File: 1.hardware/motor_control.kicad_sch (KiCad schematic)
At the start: 33 parts, among them IC1 UCC27712QDRQ1, IC4 SN74HC266D, J10 MOTOR_1_UVW, J11 MOTOR_1_HALL_SENSOR, Q10 STL130N6F7, Q2 STL130N6F7, Q3 STL130N6F7, Q4 STL130N6F7, Q8 STL130N6F7, Q9 STL130N6F7, U13 IR2101, U14 IR2101, U7 LM2904D, U8 LM2904D

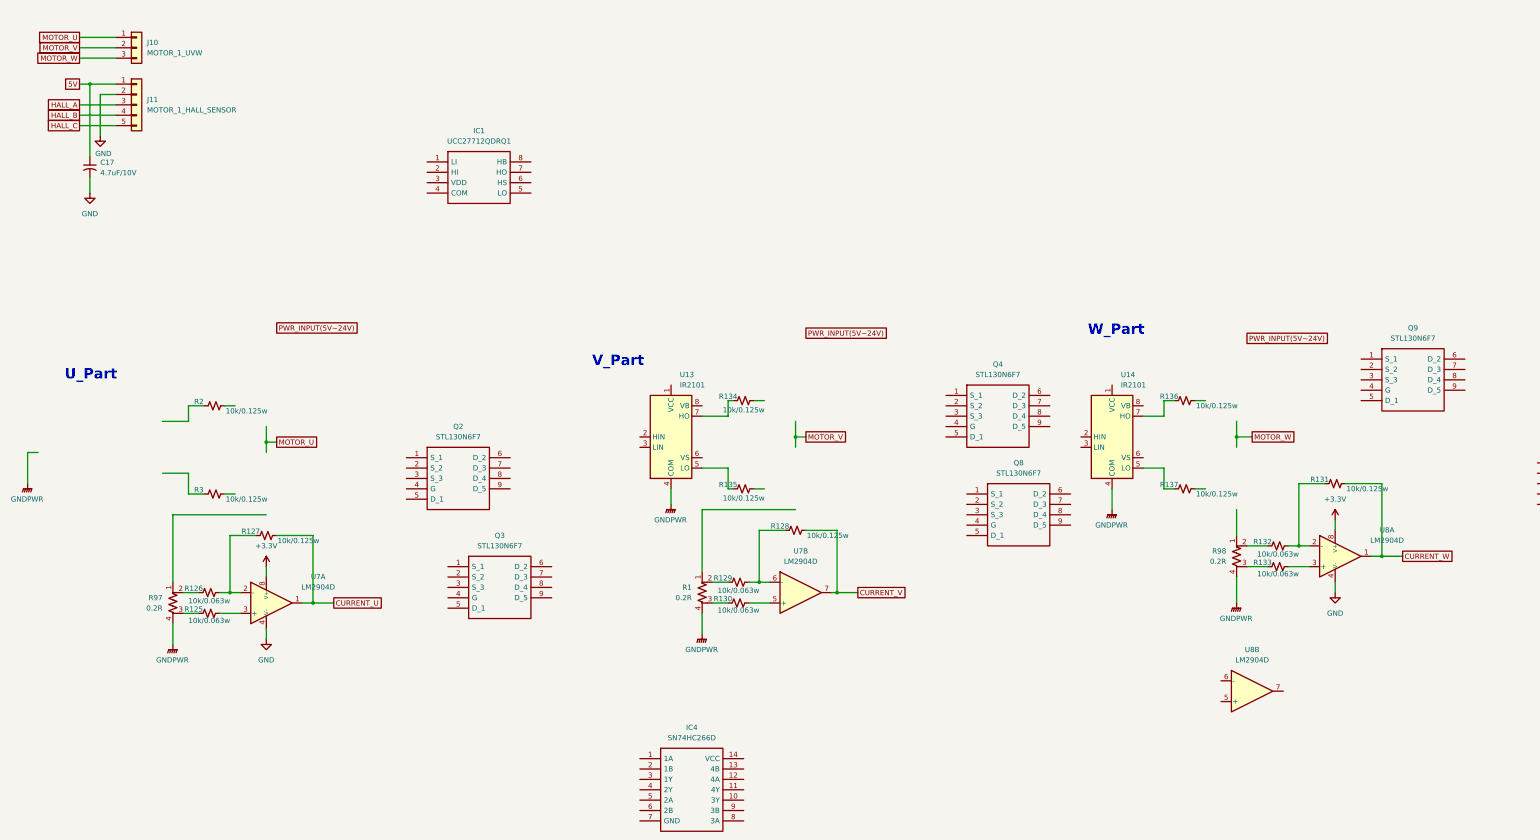
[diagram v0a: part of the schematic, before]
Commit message: 중간 저장
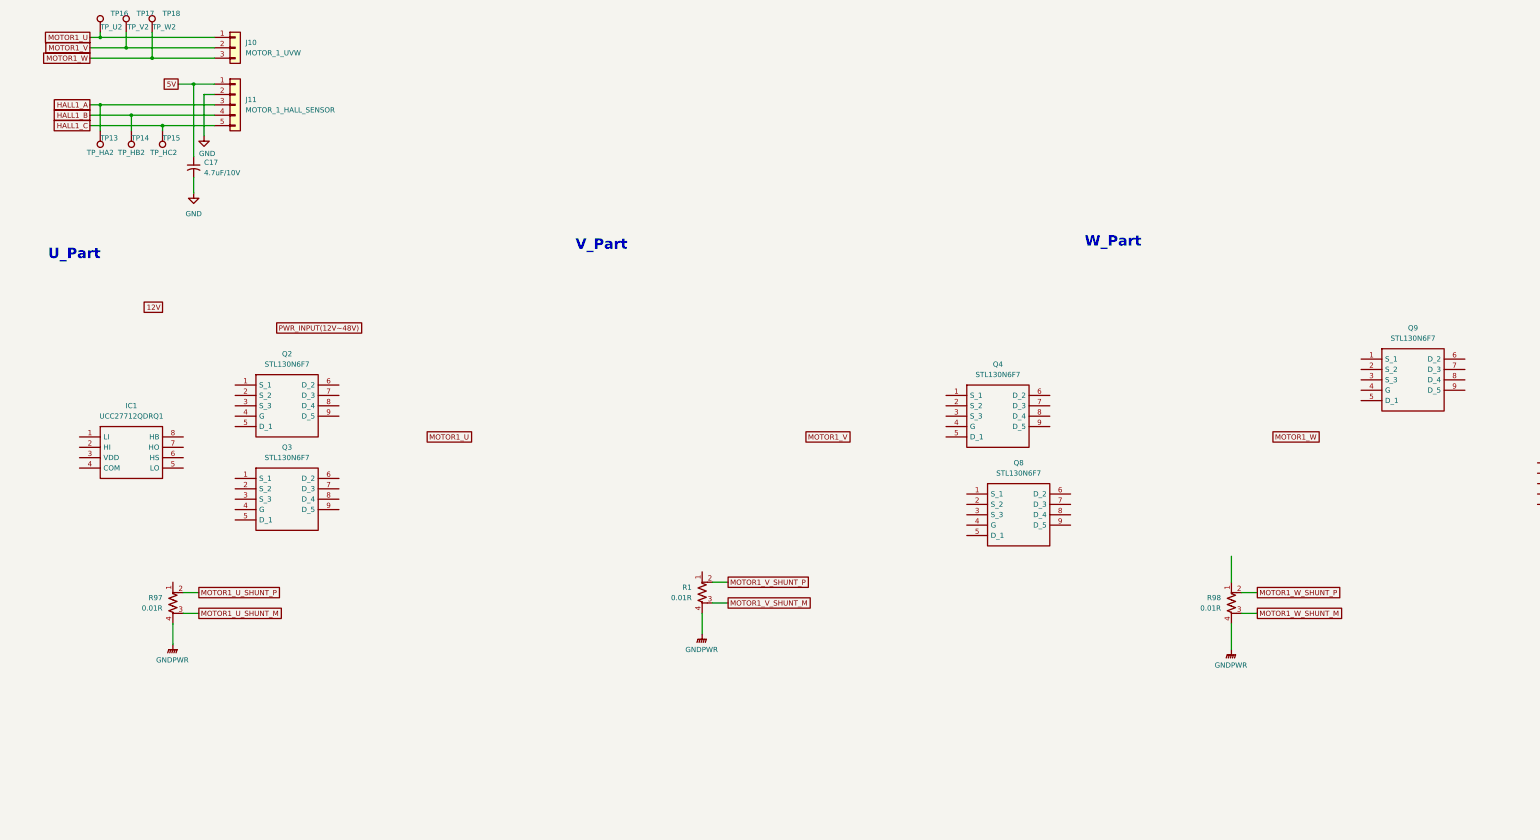
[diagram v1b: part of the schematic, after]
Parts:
- removed IC4: SN74HC266D, SOIC127P600X175-14N, symbol SamacSys_Parts:SN74HC266D
- removed R125, R126, R129, R130, R132, R133: 10k/0.063w, symbol Device:R_Small_US
- removed R127, R128, R131, R134, R135, R136, R137, R2, R3: 10k/0.125w, symbol Device:R_Small_US
- removed U13, U14: IR2101, symbol Driver_FET:IR2101
- removed U7, U8: LM2904D, PCM_Package_SO_AKL:SO-8_3.9x4.9mm_P1.27mm, symbol PCM_Amplifier_Operational_AKL:LM2904D
- added TP13: TP_HA2, symbol Connector:TestPoint
- added TP14: TP_HB2, symbol Connector:TestPoint
- added TP15: TP_HC2, symbol Connector:TestPoint
- added TP16: TP_U2, symbol Connector:TestPoint
- added TP17: TP_V2, symbol Connector:TestPoint
- added TP18: TP_W2, symbol Connector:TestPoint
- R1, R97, R98: value 0.2R -> 0.01R
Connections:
- net MOTOR1_W_SHUNT_P: now reaches R98.2
- net MOTOR1_W_SHUNT_M: now reaches R98.3
- net MOTOR1_U_SHUNT_P: now reaches R97.2
- net MOTOR1_U_SHUNT_M: now reaches R97.3
- net MOTOR1_V_SHUNT_P: now reaches R1.2
- net MOTOR1_V_SHUNT_M: now reaches R1.3
- net HALL_A renamed HALL1_A
- net HALL1_A: now also TP13.1
- net HALL_B renamed HALL1_B
- net HALL1_B: now also TP14.1
- net HALL_C renamed HALL1_C
- net HALL1_C: now also TP15.1
- net MOTOR_U renamed MOTOR1_U
- net MOTOR1_U: now also TP16.1
- net MOTOR_V renamed MOTOR1_V
- net MOTOR1_V: now also TP17.1
- net MOTOR_W renamed MOTOR1_W
- net MOTOR1_W: now also TP18.1
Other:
- moved on the sheet: C17, IC1, J10, J11, Q2, Q3, R98
